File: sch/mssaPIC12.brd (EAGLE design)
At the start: 60 x 25 mm, 30 parts, among them IC1 PIC12F675P, IC2 7805L, Q1 BC550C, Q2 BC550C

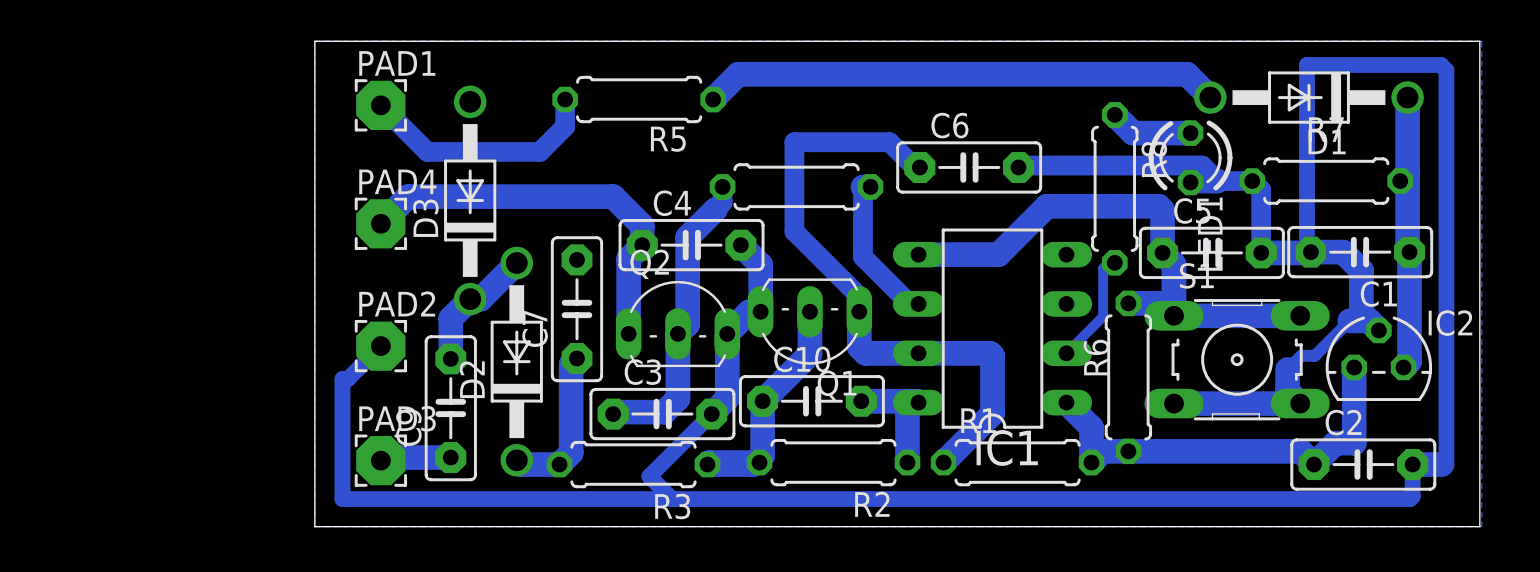
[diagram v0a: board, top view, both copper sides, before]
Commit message: SSA v.034
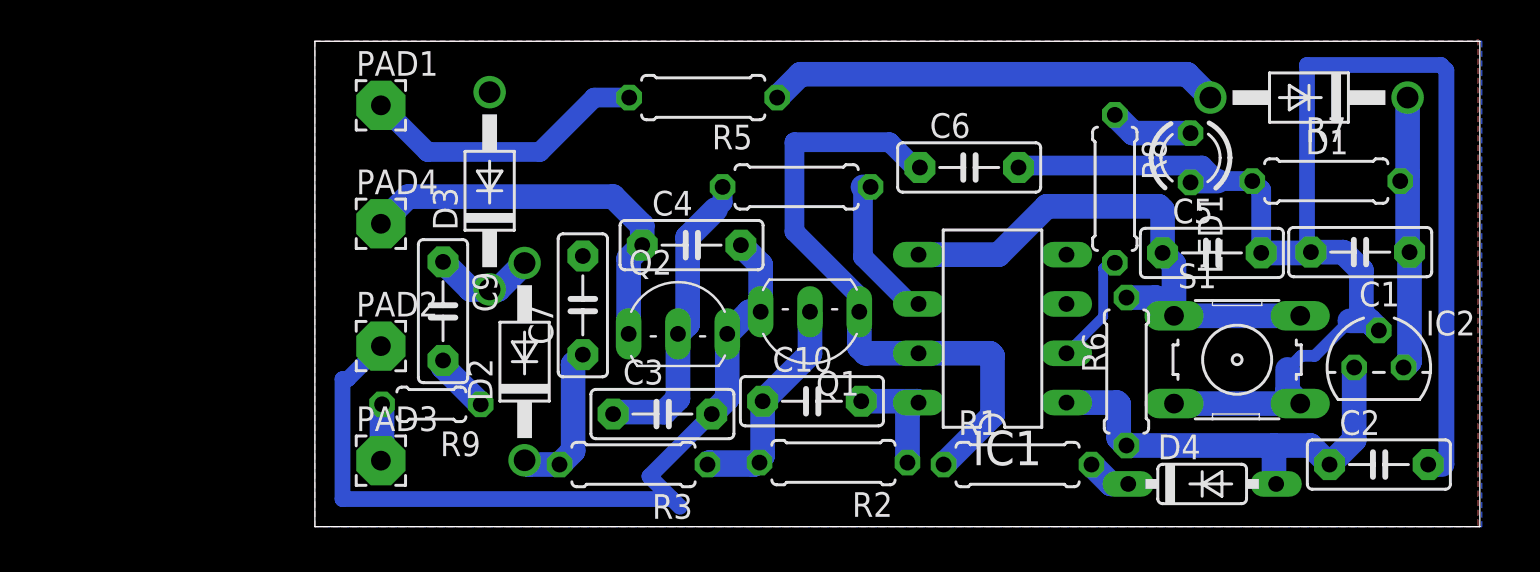
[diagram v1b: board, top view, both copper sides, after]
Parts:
- added D4: 1N4148DO35-7, diode:DO35-7
- added R9: 100, rcl:0204/5
- moved C9 5.02 mm to (6.60, 11.1), turned to 270 degrees
- moved R5 3.30 mm to (20.0, 22.1)
- moved D3 1.12 mm to (9.00, 17.3)
- moved C2 0.80 mm to (54.8, 3.20)
- moved D2 0.40 mm to (10.8, 8.50)
- moved C7 0.36 mm to (13.8, 11.4)
- moved R6 0.32 mm to (41.8, 7.99)
- moved R1 0.10 mm to (36.2, 3.20)
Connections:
- new net N$11: D4.C, R1.2
- new net N$16: PAD3.1, R9.2
- net N$13: now also C9.1; no longer C9.2
- net N$2: now also D4.A; no longer R1.2
- net N$9: now also C9.2, R9.1; no longer C9.1, PAD3.1
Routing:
- net GND: track 169.0 -> 128.9 mm
- net N$10: track 26.6 -> 23.3 mm
- net N$16: track 0.00 -> 2.92 mm
- net N$5: track 12.4 -> 14.9 mm
- net N$11: track 0.00 -> 2.30 mm
- net N$2: track 22.0 -> 23.4 mm
- net N$13: track 6.66 -> 5.35 mm
- net N$9: track 3.67 -> 3.06 mm
- added copper zone on layer 1, net GND

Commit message: Add files via upload
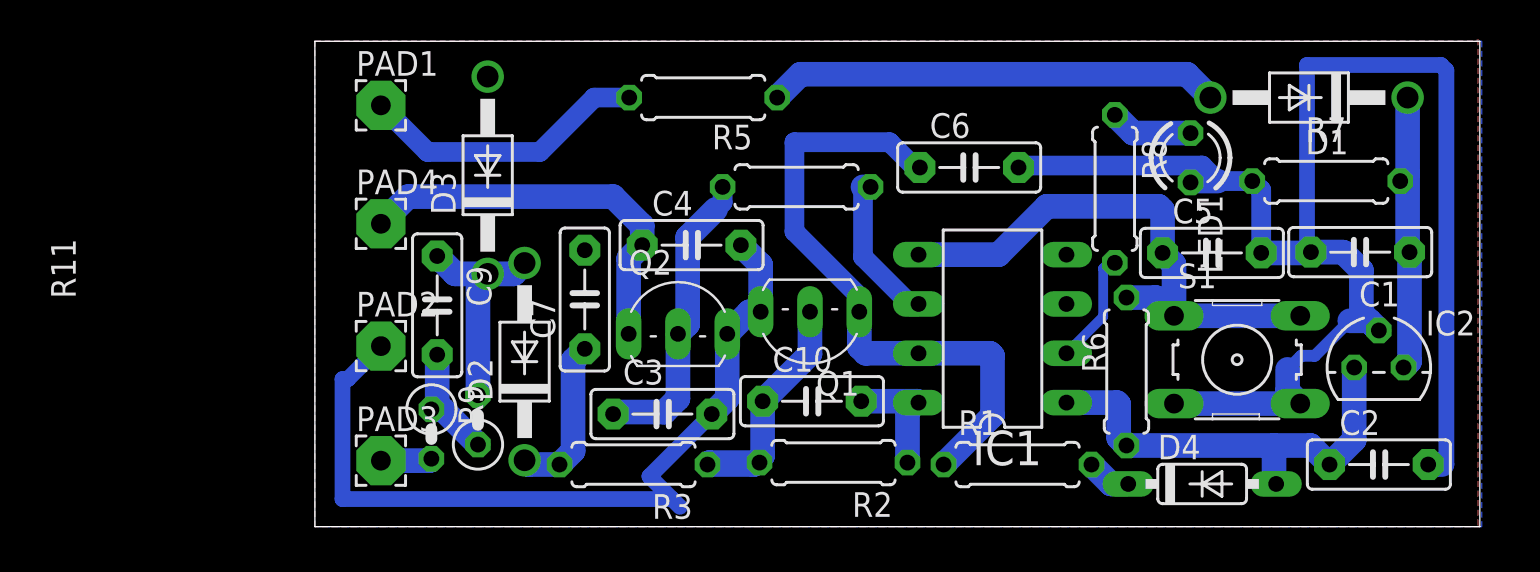
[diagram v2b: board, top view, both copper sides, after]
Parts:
- added R11: 33k, rcl:0207/2V
- R1: value 15k -> 10k
- R9: device rcl:0204/5 -> rcl:0207/2V
- moved R9 1.53 mm to (6.00, 4.77), turned to 270 degrees
- moved D3 0.81 mm to (8.90, 18.1)
- moved C9 0.42 mm to (6.30, 11.4)
- moved C7 0.32 mm to (13.9, 11.7)
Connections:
- net N$13: now also R11.2
- net N$9: now also R11.1
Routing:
- net N$13: track 5.35 -> 11.6 mm
- net N$9: track 3.06 -> 6.09 mm
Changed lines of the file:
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@@
 <attribute name="VALUE" x="27.54" y="13.372" size="1.27" layer="27" ratio="10" rot="R180"/>
 </element>
-<element name="R1" library="rcl" library_urn="urn:adsk.eagle:library:334" package="0207/7" package3d_urn="urn:adsk.eagle:package:23493/2" value="15k" x="36.19" y="3.2" smashed="yes">
+<element name="R1" library="rcl" library_urn="urn:adsk.eagle:library:334" package="0207/7" package3d_urn="urn:adsk.eagle:package:23493/2" value="10k" x="36.19" y="3.2" smashed="yes">
 <attribute name="NAME" x="33.142" y="4.724" size="1.27" layer="25" ratio="10"/>
 <attribute name="POPULARITY" value="46" x="36.19" y="3.2" size="1.778" layer="27" display="off"/>
@@
 <attribute name="VALUE" x="31.668" y="15.706" size="1.27" layer="27" ratio="10"/>
 </element>
-<element name="C7" library="capacitor-wima" package="C5B2.5" value="220n" x="13.8" y="11.4" smashed="yes" rot="R90">
-<attribute name="NAME" x="12.276" y="9.368" size="1.27" layer="25" ratio="10" rot="R90"/>
-<attribute name="VALUE" x="16.594" y="9.368" size="1.27" layer="27" ratio="10" rot="R90"/>
+<element name="C7" library="capacitor-wima" package="C5B2.5" value="220n" x="13.9" y="11.7" smashed="yes" rot="R90">
+<attribute name="NAME" x="12.376" y="9.668" size="1.27" layer="25" ratio="10" rot="R90"/>
+<attribute name="VALUE" x="16.694" y="9.668" size="1.27" layer="27" ratio="10" rot="R90"/>
 </element>
 <element name="D2" library="diode" library_urn="urn:adsk.eagle:library:210" package="DO41-10" package3d_urn="urn:adsk.eagle:package:43336/1" value="1N4004" x="10.8" y="8.5" smashed="yes" rot="R90">
@@
 <attribute name="VALUE" x="13.594" y="6.468" size="1.27" layer="27" ratio="10" rot="R90"/>
 </element>
-<element name="D3" library="diode" library_urn="urn:adsk.eagle:library:210" package="DO41-10" package3d_urn="urn:adsk.eagle:package:43336/1" value="1N4004" x="9" y="17.3" smashed="yes" rot="R90">
-<attribute name="NAME" x="7.349" y="15.268" size="1.27" layer="25" ratio="10" rot="R90"/>
-<attribute name="POPULARITY" value="82" x="9" y="17.3" size="1.778" layer="27" rot="R90" display="off"/>
-<attribute name="VALUE" x="11.794" y="15.268" size="1.27" layer="27" ratio="10" rot="R90"/>
-</element>
-<element name="C9" library="capacitor-wima" package="C5B2.5" value="220n" x="6.6" y="11.1" smashed="yes" rot="R270">
-<attribute name="NAME" x="8.124" y="13.132" size="1.27" layer="25" ratio="10" rot="R270"/>
-<attribute name="VALUE" x="3.806" y="13.132" size="1.27" layer="27" ratio="10" rot="R270"/>
+<element name="D3" library="diode" library_urn="urn:adsk.eagle:library:210" package="DO41-10" package3d_urn="urn:adsk.eagle:package:43336/1" value="1N4004" x="8.9" y="18.1" smashed="yes" rot="R90">
+<attribute name="NAME" x="7.249" y="16.068" size="1.27" layer="25" ratio="10" rot="R90"/>
+<attribute name="POPULARITY" value="82" x="8.9" y="18.1" size="1.778" layer="27" rot="R90" display="off"/>
+<attribute name="VALUE" x="11.694" y="16.068" size="1.27" layer="27" ratio="10" rot="R90"/>
+</element>
+<element name="C9" library="capacitor-wima" package="C5B2.5" value="220n" x="6.3" y="11.4" smashed="yes" rot="R270">
+<attribute name="NAME" x="7.824" y="13.432" size="1.27" layer="25" ratio="10" rot="R270"/>
+<attribute name="VALUE" x="3.506" y="13.432" size="1.27" layer="27" ratio="10" rot="R270"/>
 </element>
 <element name="R7" library="rcl" library_urn="urn:adsk.eagle:library:334" package="0207/7" package3d_urn="urn:adsk.eagle:package:23493/2" value="15k" x="52.09" y="17.8" smashed="yes">
@@
 <attribute name="VALUE" x="43.449" y="17.095" size="1.27" layer="27" ratio="10" rot="R270"/>
 </element>
-<element name="R9" library="rcl" library_urn="urn:adsk.eagle:library:334" package="0204/5" package3d_urn="urn:adsk.eagle:package:23488/1" value="100" x="6" y="6.3" smashed="yes" rot="R180">
-<attribute name="NAME" x="8.54" y="4.903" size="1.27" layer="25" ratio="10" rot="R180"/>
-<attribute name="POPULARITY" value="35" x="6" y="6.3" size="1.778" layer="27" rot="R180" display="off"/>
-<attribute name="SPICEPREFIX" value="R" x="6" y="6.3" size="1.778" layer="27" rot="R180" display="off"/>
-<attribute name="VALUE" x="8.286" y="6.8588" size="1.27" layer="27" ratio="10" rot="R180"/>
+<element name="R9" library="rcl" library_urn="urn:adsk.eagle:library:334" package="0207/2V" package3d_urn="urn:adsk.eagle:package:23490/1" value="100" x="6" y="4.77" smashed="yes" rot="R270">
+<attribute name="NAME" x="7.397" y="7.31" size="1.27" layer="25" ratio="10" rot="R270"/>
+<attribute name="POPULARITY" value="17" x="6" y="4.77" size="1.778" layer="27" rot="R270" display="off"/>
+<attribute name="SPICEPREFIX" value="R" x="6" y="4.77" size="1.778" layer="27" rot="R270" display="off"/>
+<attribute name="VALUE" x="5.4412" y="7.056" size="1.27" layer="27" ratio="10" rot="R270"/>
 </element>
 <element name="D4" library="diode" library_urn="urn:adsk.eagle:library:210" package="DO35-7" package3d_urn="urn:adsk.eagle:package:43339/2" value="1N4148DO35-7" x="45.7" y="2.2" smashed="yes">
@@
 <attribute name="POPULARITY" value="58" x="45.7" y="2.2" size="1.778" layer="27" display="off"/>
 <attribute name="VALUE" x="43.414" y="-0.467" size="1.27" layer="27" ratio="10"/>
+</element>
+<element name="R11" library="rcl" library_urn="urn:adsk.eagle:library:334" package="0207/2V" package3d_urn="urn:adsk.eagle:package:23490/1" value="33k" x="8.4" y="5.5" smashed="yes" rot="R90">
+<attribute name="NAME" x="-12.316" y="11.7492" size="1.27" layer="25" ratio="10" rot="R90"/>
+<attribute name="POPULARITY" value="17" x="8.4" y="5.5" size="1.778" layer="27" rot="R90" display="off"/>
+<attribute name="SPICEPREFIX" value="R" x="8.4" y="5.5" size="1.778" layer="27" rot="R90" display="off"/>
+<attribute name="VALUE" x="10.6352" y="5.4492" size="1.27" layer="27" ratio="10" rot="R90"/>
 </element>
 </elements>
@@
 <contactref element="R3" pad="2"/>
 <contactref element="D2" pad="C"/>
-<wire x1="13.8" y1="8.86" x2="13.3" y2="8.36" width="1.27" layer="16"/>
-<wire x1="13.3" y1="8.36" x2="13.3" y2="3.9" width="1.27" layer="16"/>
+<wire x1="13.9" y1="9.16" x2="13.3" y2="8.56" width="1.27" layer="16"/>
+<wire x1="13.3" y1="8.56" x2="13.3" y2="3.9" width="1.27" layer="16"/>
 <wire x1="13.3" y1="3.9" x2="12.6" y2="3.2" width="1.27" layer="16"/>
 <wire x1="12.6" y1="3.2" x2="11.02" y2="3.2" width="1.27" layer="16"/>
@@
 <contactref element="D3" pad="C"/>
 <contactref element="D2" pad="A"/>
-<wire x1="10.8" y1="13.58" x2="9.44" y2="12.22" width="1.27" layer="16"/>
-<wire x1="9.44" y1="12.22" x2="9" y2="12.22" width="1.27" layer="16"/>
+<wire x1="10.8" y1="13.58" x2="10.24" y2="13.02" width="1.27" layer="16"/>
+<wire x1="10.24" y1="13.02" x2="8.9" y2="13.02" width="1.27" layer="16"/>
 <contactref element="C9" pad="1"/>
-<wire x1="6.6" y1="13.64" x2="8.02" y2="12.22" width="1.27" layer="16"/>
-<wire x1="8.02" y1="12.22" x2="9" y2="12.22" width="1.27" layer="16"/>
+<wire x1="6.3" y1="13.94" x2="7.22" y2="13.02" width="1.27" layer="16"/>
+<wire x1="7.22" y1="13.02" x2="8.9" y2="13.02" width="1.27" layer="16"/>
+<contactref element="R11" pad="2"/>
+<wire x1="8.4" y1="6.77" x2="8.4" y2="12.52" width="1.27" layer="16"/>
+<wire x1="8.4" y1="12.52" x2="8.9" y2="13.02" width="1.27" layer="16"/>
 </signal>
 <signal name="N$14">
@@
 <contactref element="C9" pad="2"/>
 <contactref element="R9" pad="1"/>
-<wire x1="8.54" y1="6.3" x2="6.6" y2="8.24" width="1.27" layer="16"/>
-<wire x1="6.6" y1="8.24" x2="6.6" y2="8.56" width="1.27" layer="16"/>
+<contactref element="R11" pad="1"/>
+<wire x1="6.3" y1="8.86" x2="6.3" y2="6.34" width="1.27" layer="16"/>
+<wire x1="6" y1="6.04" x2="6.3" y2="6.34" width="1.27" layer="16"/>
+<wire x1="6" y1="6.04" x2="6.59" y2="6.04" width="1.27" layer="16"/>
+<wire x1="6.59" y1="6.04" x2="8.4" y2="4.23" width="1.27" layer="16"/>
 </signal>
 <signal name="N$16">
 <contactref element="R9" pad="2"/>
 <contactref element="PAD3" pad="1"/>
-<wire x1="3.46" y1="6.3" x2="3.46" y2="3.46" width="1.27" layer="16"/>
-<wire x1="3.46" y1="3.46" x2="3.4" y2="3.4" width="1.27" layer="16"/>
+<wire x1="6" y1="3.5" x2="5.9" y2="3.4" width="1.27" layer="16"/>
+<wire x1="5.9" y1="3.4" x2="3.4" y2="3.4" width="1.27" layer="16"/>
 </signal>
 <signal name="N$17">

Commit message: Add files via upload
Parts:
- C7: value 220n -> 470n
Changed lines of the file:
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@@
 <attribute name="VALUE" x="31.668" y="15.706" size="1.27" layer="27" ratio="10"/>
 </element>
-<element name="C7" library="capacitor-wima" package="C5B2.5" value="220n" x="13.9" y="11.7" smashed="yes" rot="R90">
+<element name="C7" library="capacitor-wima" package="C5B2.5" value="470n" x="13.9" y="11.7" smashed="yes" rot="R90">
 <attribute name="NAME" x="12.376" y="9.668" size="1.27" layer="25" ratio="10" rot="R90"/>
 <attribute name="VALUE" x="16.694" y="9.668" size="1.27" layer="27" ratio="10" rot="R90"/>
